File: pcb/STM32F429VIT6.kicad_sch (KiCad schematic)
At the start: 13 parts, among them U2 STM32F429VITx

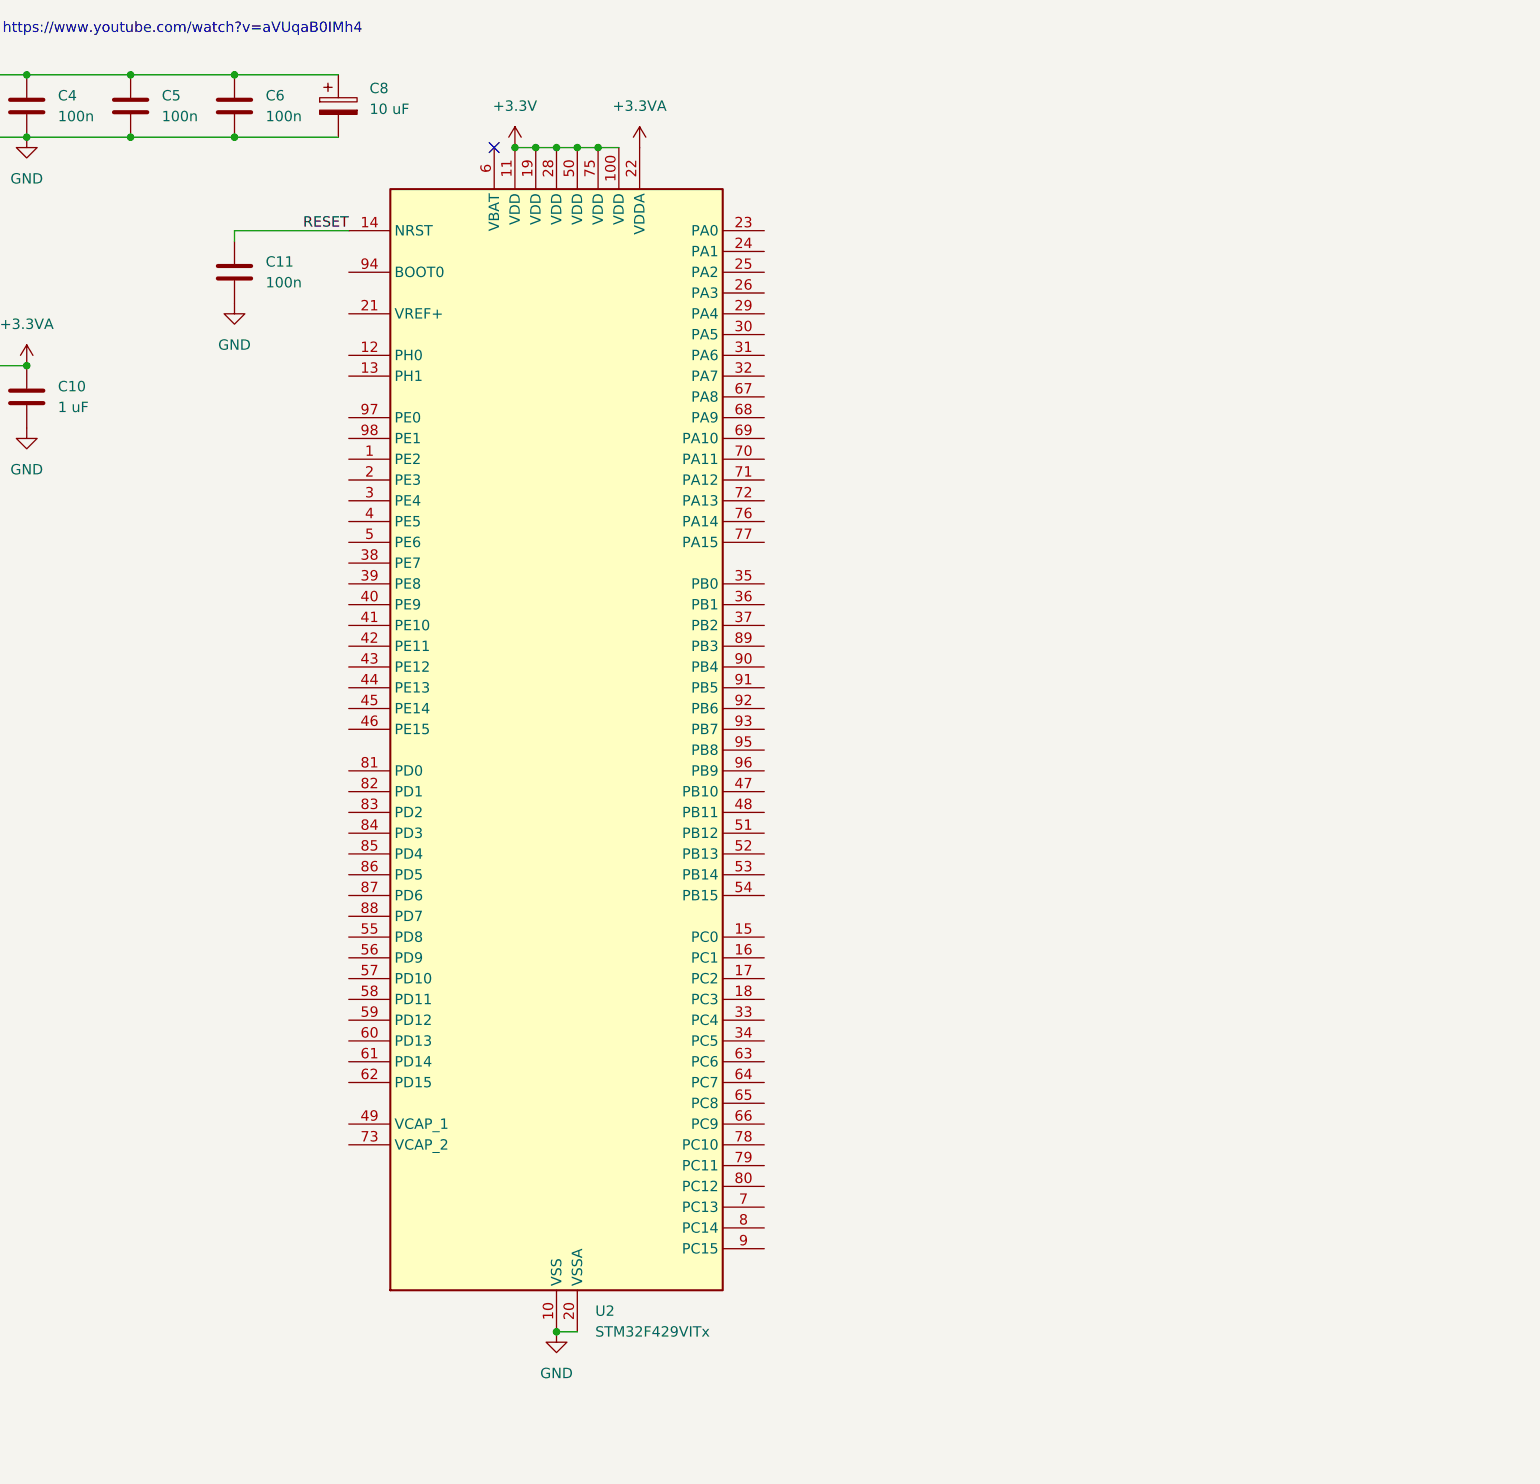
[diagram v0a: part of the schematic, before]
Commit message: ⚙️ wip, stm32 reference schem + jobset
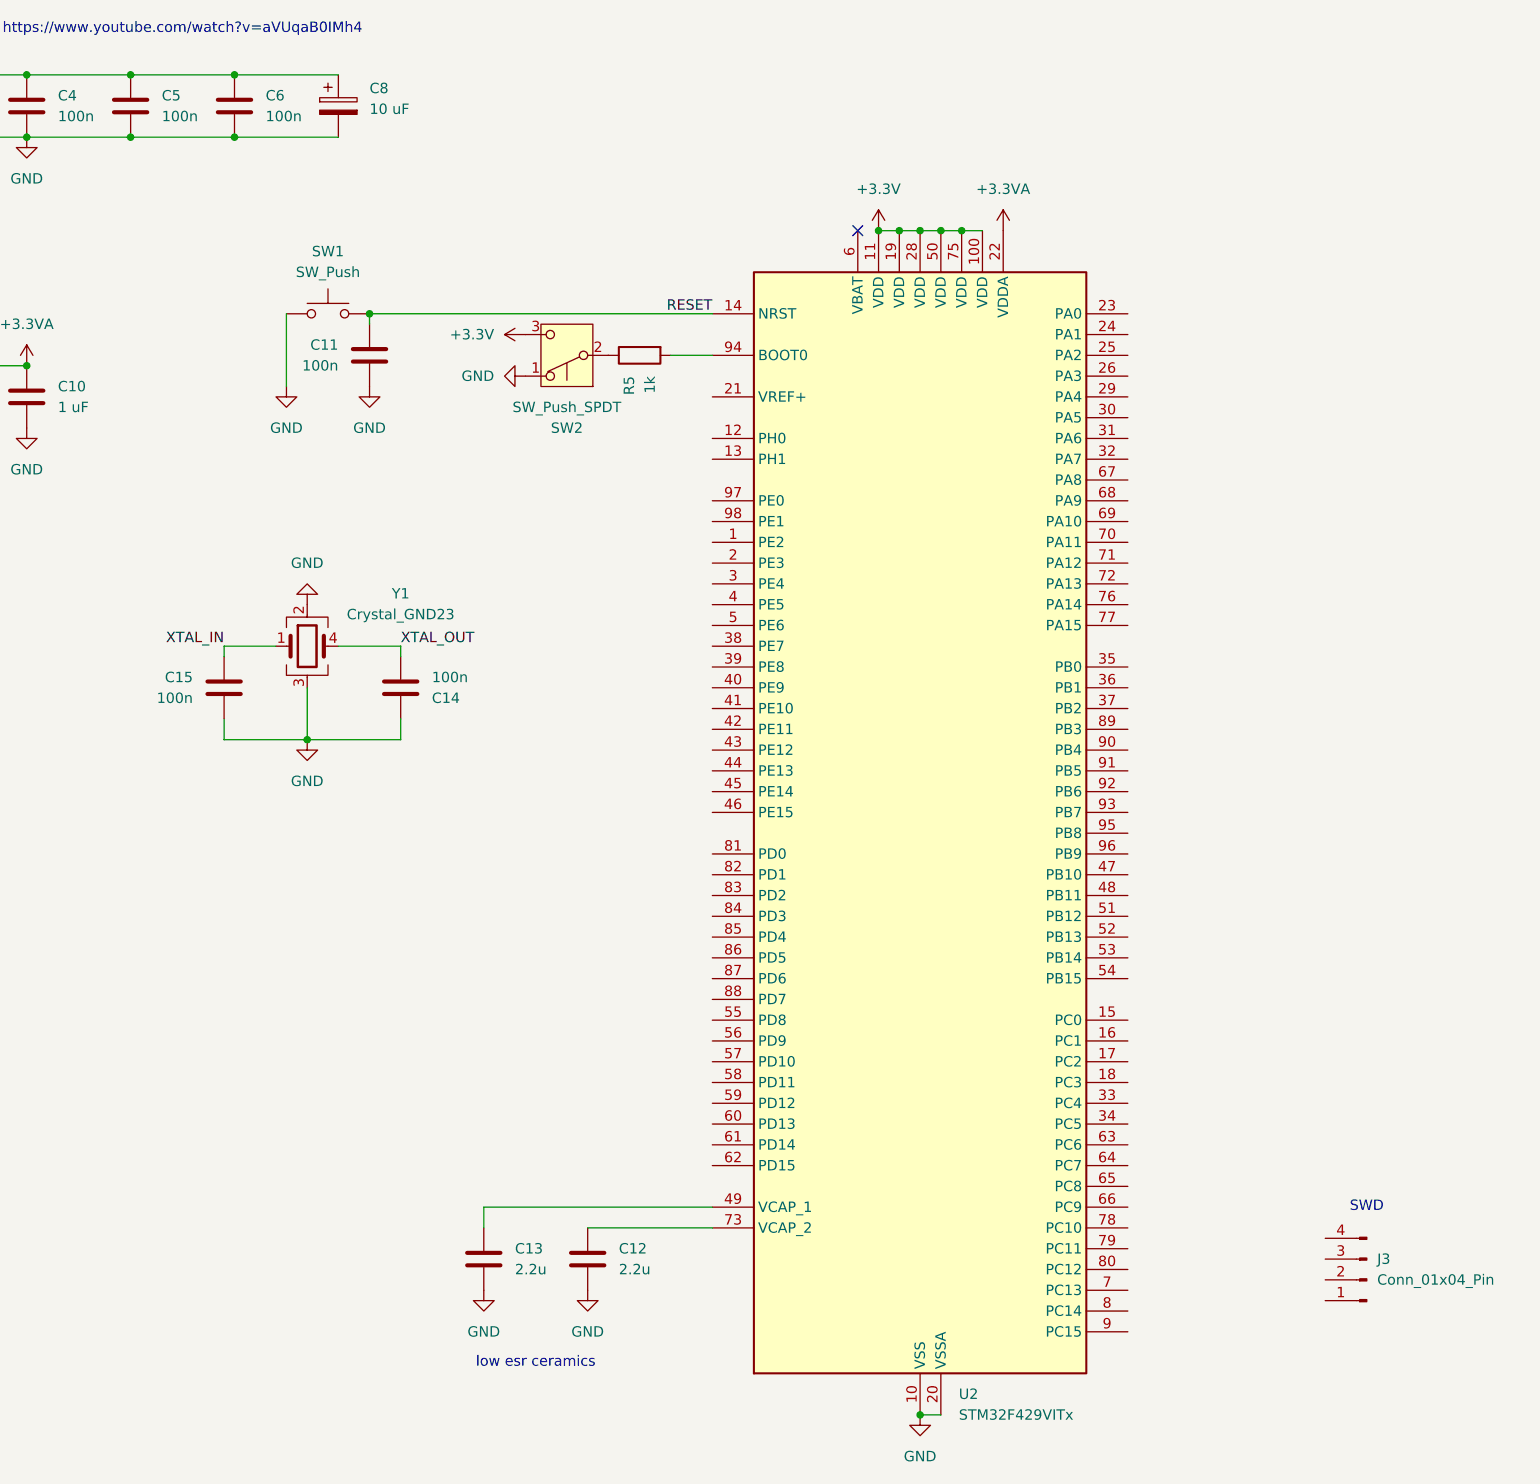
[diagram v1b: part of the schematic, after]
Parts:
- added C12, C13: 2.2u, Capacitor_SMD:C_0201_0603Metric, symbol Device:C
- added C14, C15: 100n, Capacitor_SMD:C_0201_0603Metric, symbol Device:C
- added J3: Conn_01x04_Pin, symbol Connector:Conn_01x04_Pin
- added R5: 1k, symbol Device:R
- added SW1: SW_Push, symbol Switch:SW_Push
- added SW2: SW_Push_SPDT, symbol Switch:SW_Push_SPDT
- added Y1: Crystal_GND23, Crystal:Crystal_SMD_2520-4Pin_2.5x2.0mm, symbol Device:Crystal_GND23
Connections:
- net +3.3V: now also SW2.3 (C)
- net GND: now also C12.2, C13.2, C14.1, C15.2, SW1.1, SW2.1 (A), Y1.2, Y1.3
- net RESET: now also SW1.2
- net at U2.49 (VCAP_1): now also C13.1
- net at U2.73 (VCAP_2): now also C12.1
- net at U2.94 (BOOT0): now also R5.2
- new net: R5.1, SW2.2 (B)
- new net XTAL_IN: C15.1, Y1.1
- new net XTAL_OUT: C14.2, Y1.4
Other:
- note added: "SWD"
- note added: "low esr ceramics"
- moved on the sheet: C11, U2
